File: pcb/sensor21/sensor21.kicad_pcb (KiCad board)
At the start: 2 copper layers, 83.5 x 66.2 mm, 34 parts, among them IC1 ATMEGA8-P, P1 nRF24L01, P2 BME280, P3 CONN_01X02, Q1 BC548, U1 LM2931AZ-3.3/5.0, Y1 8Mhz

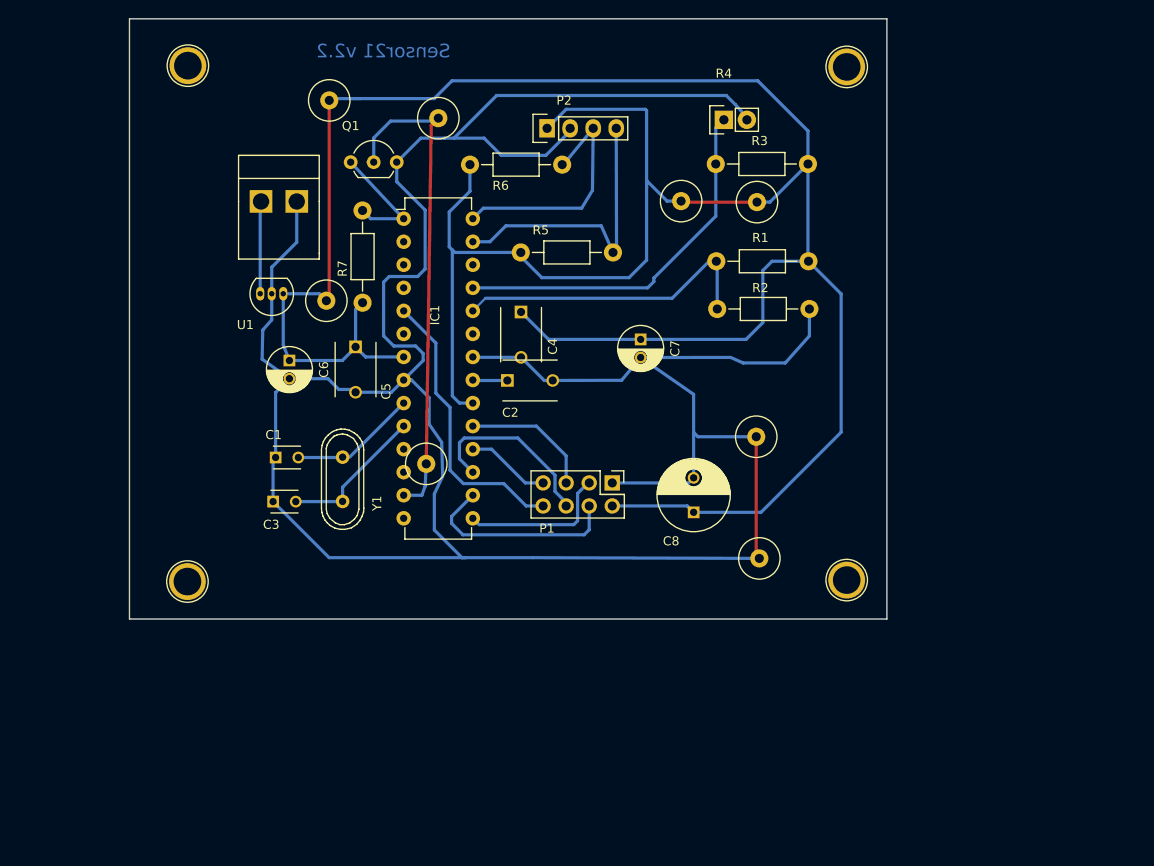
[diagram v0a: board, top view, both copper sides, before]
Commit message: all works ok
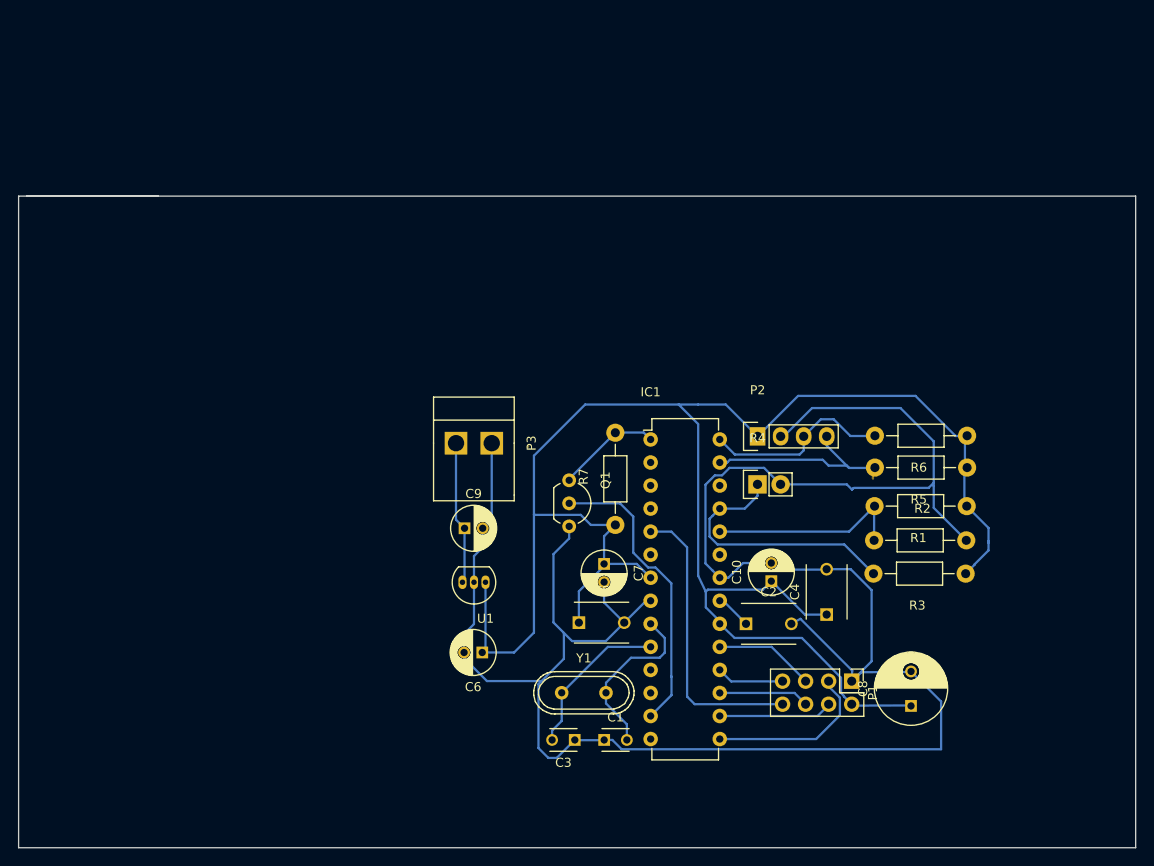
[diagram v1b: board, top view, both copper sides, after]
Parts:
- removed 1-REF**, 2-REF**, 3-REF**, 4-REF**, 5-REF**, 6-REF**, 7-REF**, 8-REF**, LB-REF**, LT-REF**, RB-REF**, RT-REF**: 1pin, Connect:1pin
- added C10: 10u, Capacitors_ThroughHole:C_Radial_D5_L11_P2, F.Cu at (155.6, 102.9)
- added C9: 10u, Capacitors_ThroughHole:C_Radial_D5_L11_P2, F.Cu at (121.7, 97.0)
- U1: value LM2931AZ-3.3/5.0 -> HT7333
- moved R6 62.4 mm to (177.1, 86.8), turned to 180 degrees
- moved R5 54.6 mm to (177.1, 90.3), turned to 180 degrees
- moved R3 48.4 mm to (177.0, 102.0)
- moved C1 47.8 mm to (137.1, 120.4)
- moved C4 47.4 mm to (161.7, 106.5), turned to 90 degrees
- moved Q1 42.5 mm to (133.3, 91.8), turned to 270 degrees
- moved C3 42.4 mm to (133.9, 120.4), turned to 180 degrees
- moved P2 41.1 mm to (154.0, 86.9)
- moved R4 40.4 mm to (154.0, 92.2)
- moved C5 39.1 mm to (134.3, 107.4), turned to 0 degrees
- moved U1 38.8 mm to (124.0, 103.0)
- moved C6 38.6 mm to (123.7, 110.7), turned to 180 degrees
- moved C2 37.6 mm to (152.8, 107.6)
- moved R7 37.1 mm to (138.4, 96.7)
- moved IC1 36.5 mm to (142.2, 87.2)
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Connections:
- IC1 pad 11: Net-(IC1-Pad11) -> (no net)
- IC1 pad 12: Net-(IC1-Pad12) -> (no net)
- IC1 pad 14: Net-(IC1-Pad14) -> (no net)
- IC1 pad 2: Net-(IC1-Pad2) -> (no net)
- IC1 pad 23: Net-(IC1-Pad23) -> (no net)
- IC1 pad 26: Net-(IC1-Pad26) -> (no net)
- IC1 pad 3: Net-(IC1-Pad3) -> (no net)
- IC1 pad 4: Net-(IC1-Pad4) -> (no net)
- IC1 pad 6: Net-(IC1-Pad6) -> (no net)
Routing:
- net +3V3: track 317.2 -> 202.6 mm
- net GND: track 311.7 -> 254.4 mm
- net PD7: track 55.5 -> 32.9 mm
- net PC1: track 34.4 -> 22.2 mm
- net PC2: track 41.3 -> 29.6 mm
- net MOSI: track 20.6 -> 10.1 mm
- net CSN: track 22.9 -> 12.7 mm
- net SDA: track 31.9 -> 23.9 mm
- net SCL: track 27.0 -> 21.0 mm
- net Net-(C9-Pad1): track 10.2 -> 15.8 mm
- net Net-(C1-Pad2): track 14.1 -> 19.4 mm
- net SCK: track 14.6 -> 11.2 mm
- net MISO: track 9.66 -> 7.58 mm
- net CE: track 16.8 -> 18.7 mm
- net RESET: track 13.4 -> 11.9 mm
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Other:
- board size 83.5 x 66.2 mm -> 123.1 x 71.8 mm
- net class moje removed
- rule pad_to_mask_clearance: 0.2 -> 0
- board text removed: "Sensor21 v2.2"
